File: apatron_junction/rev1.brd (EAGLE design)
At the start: 48 x 24 mm, 47 parts, among them IC1 MCP1703CB, U1 STM32F030K6T6

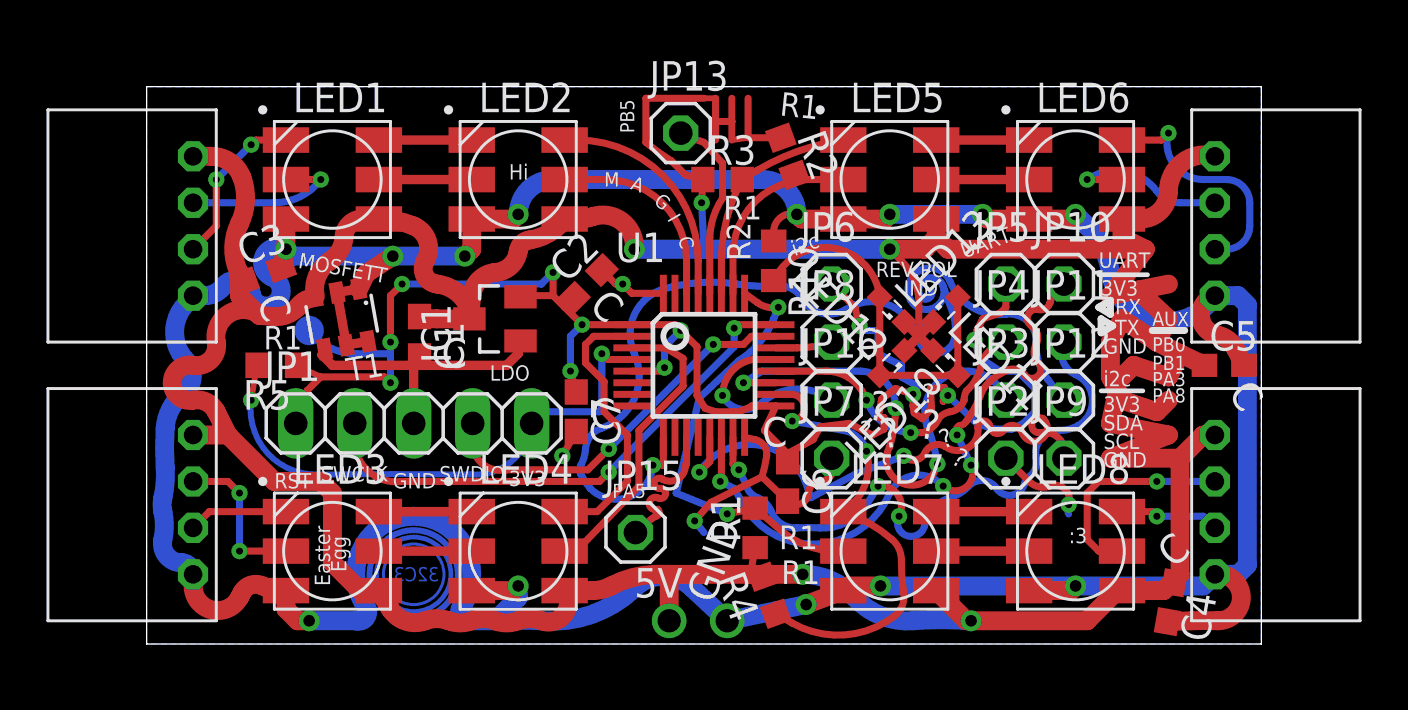
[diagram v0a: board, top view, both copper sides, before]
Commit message: Rev1 production
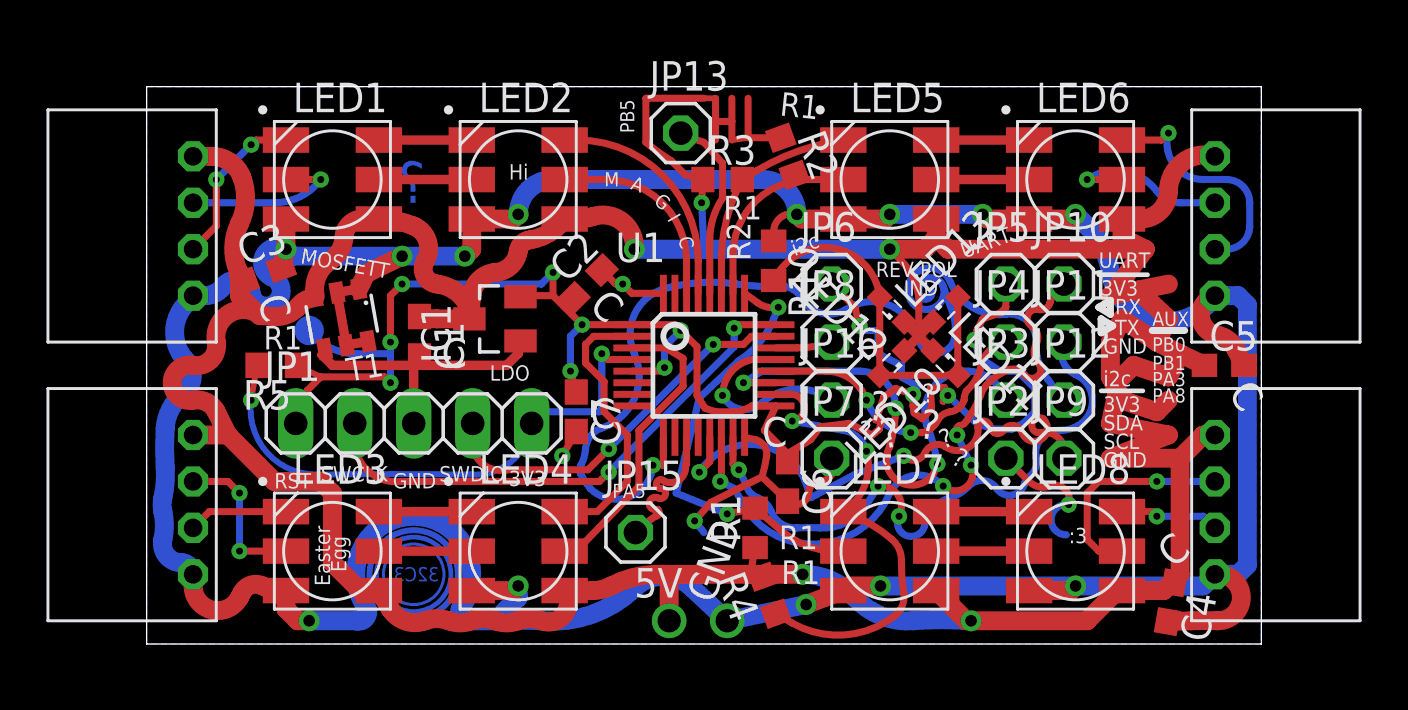
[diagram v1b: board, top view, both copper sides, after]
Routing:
- net GND: track 31.9 -> 32.8 mm
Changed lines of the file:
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@@
 <layer number="18" name="Vias" color="2" fill="1" visible="yes" active="yes"/>
 <layer number="19" name="Unrouted" color="6" fill="1" visible="yes" active="yes"/>
-<layer number="20" name="Dimension" color="15" fill="1" visible="yes" active="yes"/>
-<layer number="21" name="tPlace" color="7" fill="1" visible="yes" active="yes"/>
-<layer number="22" name="bPlace" color="7" fill="1" visible="yes" active="yes"/>
-<layer number="23" name="tOrigins" color="15" fill="1" visible="yes" active="yes"/>
-<layer number="24" name="bOrigins" color="15" fill="1" visible="yes" active="yes"/>
+<layer number="20" name="Dimension" color="15" fill="1" visible="no" active="yes"/>
+<layer number="21" name="tPlace" color="7" fill="1" visible="no" active="yes"/>
+<layer number="22" name="bPlace" color="7" fill="1" visible="no" active="yes"/>
+<layer number="23" name="tOrigins" color="15" fill="1" visible="no" active="yes"/>
+<layer number="24" name="bOrigins" color="15" fill="1" visible="no" active="yes"/>
 <layer number="25" name="tNames" color="7" fill="1" visible="no" active="yes"/>
 <layer number="26" name="bNames" color="7" fill="1" visible="no" active="yes"/>
@@
 <text x="19.1" y="9.3" size="1.27" layer="21" font="vector">C</text>
 <text x="26" y="16.5" size="1.016" layer="21" font="vector" ratio="10" rot="R90">R2</text>
-<text x="6.5" y="16.2" size="0.6604" layer="21" font="vector" ratio="20" rot="R350">MOSFETT</text>
+<text x="6.6" y="16.4" size="0.6604" layer="21" font="vector" ratio="20" rot="R350">MOSFETT</text>
 <text x="16.5" y="12" size="0.6604" layer="21" font="vector" ratio="20" rot="R180">LDO</text>
 <text x="43.5" y="16.5" size="6.4516" layer="22" font="vector" ratio="16" rot="MR0">APATRON</text>
@@
 <circle x="4.9" y="13" radius="0.762" width="0" layer="30"/>
 <text x="5.1" y="14.6" size="0.6604" layer="22" font="vector" ratio="16" rot="MR310">GNDD</text>
+<text x="12" y="19" size="1.778" layer="16" font="vector" rot="MR0">?</text>
 </plain>
 <attributes>
@@
 <wire x1="38.9" y1="6.8" x2="39.7" y2="6" width="0.3048" layer="1" curve="-129.884516"/>
 <via x="39.7" y="6" extent="1-16" drill="0.3"/>
-<wire x1="39.7" y1="6" x2="39.7" y2="5.6" width="0.3048" layer="16" curve="39.884403"/>
 <wire x1="27.6" y1="6.15" x2="28.5" y2="6.5" width="0.3048" layer="1" curve="129.836748"/>
 <wire x1="28.5" y1="6.5" x2="29" y2="7" width="0.3048" layer="1" curve="-82.338055"/>
 <wire x1="29" y1="7" x2="29.5" y2="8" width="0.3048" layer="1" curve="119.209933"/>
+<wire x1="39.6" y1="4.7" x2="39.7" y2="6" width="0.3048" layer="16" curve="-188.79742"/>
 </signal>
 <signal name="N$1">
@@
 <wire x1="17.5" y1="16" x2="17.5" y2="15" width="0.3048" layer="1"/>
 <contactref element="JP5" pad="1"/>
-<wire x1="31.75" y1="9.25" x2="31.75" y2="9.75" width="0.3048" layer="1"/>
-<wire x1="31.75" y1="9.75" x2="31.5" y2="9.75" width="0.3048" layer="1"/>
-<wire x1="31.5" y1="9.75" x2="31.65" y2="10.55" width="0.3048" layer="1"/>
-<wire x1="31.65" y1="10.55" x2="32.25" y2="11" width="0.3048" layer="1"/>
+<wire x1="31.55" y1="9.25" x2="31.65" y2="9.65" width="0.3048" layer="1"/>
+<wire x1="31.65" y1="9.65" x2="31.4" y2="9.65" width="0.3048" layer="1"/>
+<wire x1="31.4" y1="9.65" x2="31.75" y2="10.65" width="0.3048" layer="1"/>
+<wire x1="31.75" y1="10.65" x2="32.25" y2="11" width="0.3048" layer="1"/>
 <wire x1="32.25" y1="11" x2="33" y2="10.75" width="0.3048" layer="1"/>
 <wire x1="33" y1="10.75" x2="33" y2="10.25" width="0.3048" layer="1"/>
@@
 <wire x1="27.1" y1="10.25" x2="26.6" y2="9.2" width="0.3048" layer="1"/>
 <wire x1="26.6" y1="9.2" x2="27.6" y2="8.2" width="0.3048" layer="1"/>
-<wire x1="27.6" y1="8.2" x2="28.7" y2="8.8" width="0.3048" layer="1"/>
-<wire x1="28.7" y1="8.8" x2="29" y2="9.35" width="0.3048" layer="1"/>
+<wire x1="27.6" y1="8.2" x2="28.6" y2="8.8" width="0.3048" layer="1"/>
+<wire x1="28.6" y1="8.8" x2="29" y2="9.35" width="0.3048" layer="1"/>
 <wire x1="29" y1="9.35" x2="30.25" y2="9.5" width="0.3048" layer="1"/>
 <wire x1="30.25" y1="9.5" x2="31.25" y2="9" width="0.3048" layer="1"/>
-<wire x1="31.25" y1="9" x2="31.75" y2="9.25" width="0.3048" layer="1"/>
+<wire x1="31.25" y1="9" x2="31.55" y2="9.25" width="0.3048" layer="1"/>
 <contactref element="C6" pad="1"/>
 <wire x1="27.6" y1="7.85" x2="27.6" y2="8.2" width="0.3048" layer="1"/>
@@
 <contactref element="LED8" pad="3"/>
 <wire x1="9.135871875" y1="15.29749375" x2="9.45" y2="15.95" width="0.8128" layer="1"/>
-<wire x1="9.45" y1="15.95" x2="10.6" y2="16.7" width="0.8128" layer="1"/>
-<via x="10.6" y="16.7" extent="1-16" drill="0.5"/>
-<wire x1="10.6" y1="16.7" x2="13.7" y2="16.7" width="0.8128" layer="16"/>
+<wire x1="9.45" y1="15.95" x2="11" y2="16.7" width="0.8128" layer="1"/>
+<via x="11" y="16.7" extent="1-16" drill="0.5"/>
+<wire x1="11" y1="16.7" x2="13.7" y2="16.7" width="0.8128" layer="16"/>
 <via x="13.7" y="16.7" extent="1-16" drill="0.5"/>
 <wire x1="13.7" y1="16.7" x2="14" y2="17" width="0.8128" layer="1"/>
@@
 <via x="6" y="17" extent="1-16" drill="0.5"/>
 <wire x1="6" y1="17" x2="6.3" y2="16.7" width="0.8128" layer="16"/>
-<wire x1="6.3" y1="16.7" x2="10.6" y2="16.7" width="0.8128" layer="16"/>
+<wire x1="6.3" y1="16.7" x2="11" y2="16.7" width="0.8128" layer="16"/>
 <wire x1="46" y1="15" x2="47" y2="15" width="0.8128" layer="16"/>
 <wire x1="47" y1="15" x2="47.4" y2="14.6" width="0.8128" layer="16"/>
@@
 <contactref element="JP15" pad="1"/>
 <contactref element="U1" pad="11"/>
-<wire x1="23.2" y1="7.7" x2="22.2" y2="7.1" width="0.3048" layer="1" curve="-122.09836"/>
-<wire x1="22.2" y1="7.1" x2="22.1" y2="6.7" width="0.3048" layer="1" curve="220.896606"/>
+<wire x1="23.2" y1="7.7" x2="22.3" y2="7" width="0.3048" layer="1" curve="-122.09836"/>
+<wire x1="22.3" y1="7" x2="22.1" y2="6.7" width="0.3048" layer="1" curve="220.896606"/>
 <wire x1="22.1" y1="6.7" x2="22" y2="6.3" width="0.3048" layer="1" curve="-220.895127"/>
 <wire x1="22" y1="6.3" x2="22" y2="5.8" width="0.3048" layer="1" curve="220.894017"/>
